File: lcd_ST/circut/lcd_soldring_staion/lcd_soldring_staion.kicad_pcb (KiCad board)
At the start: 2 copper layers, 41.7 x 41 mm, 35 parts, among them J2 Conn_01x05_Pin, J3 Conn_01x01_Pin, J4 Conn_01x01_Pin, J44 Screw_Terminal_01x02, J5 Conn_01x01_Pin, J6 Conn_01x01_Pin, J7 Conn_01x04_Pin, Q2 Si4162DY, SW1 SW_Push, U1 PIC16F15223T-I/SL, U2 L7805, U3 LM358

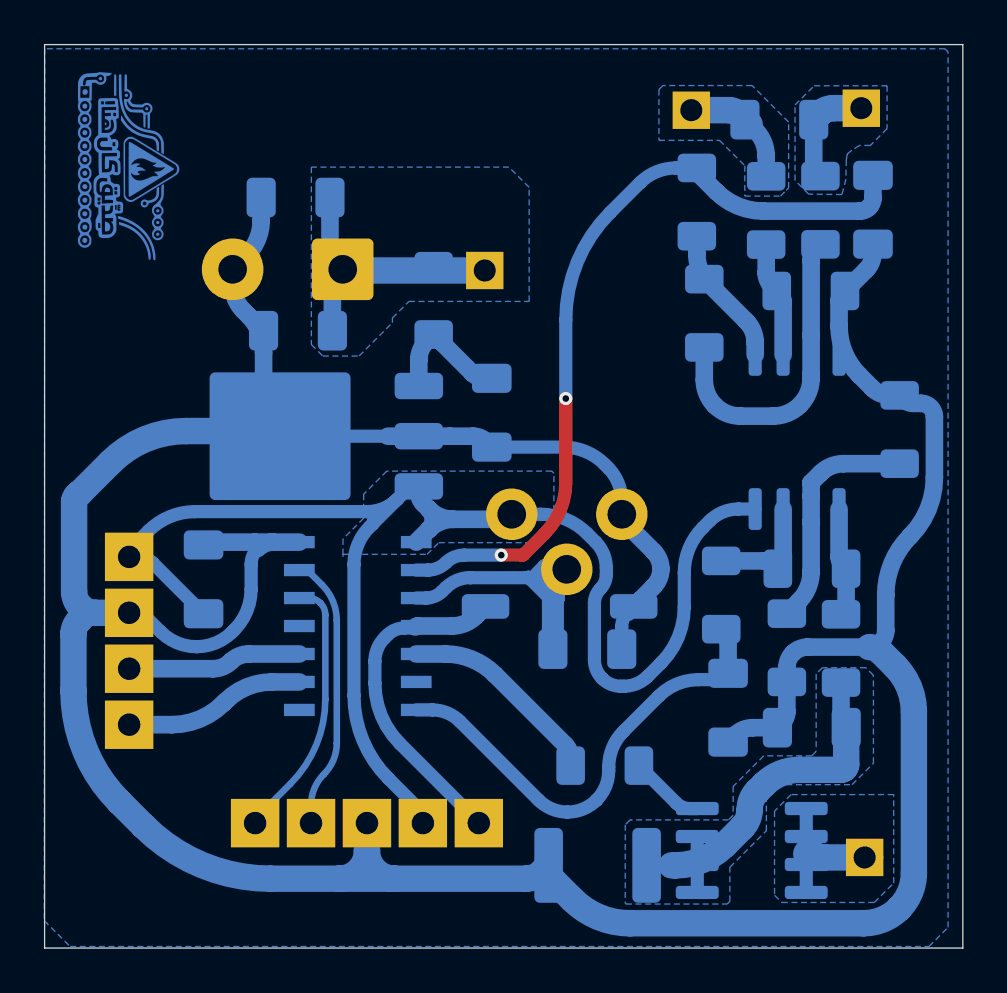
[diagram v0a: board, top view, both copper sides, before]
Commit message: done v0
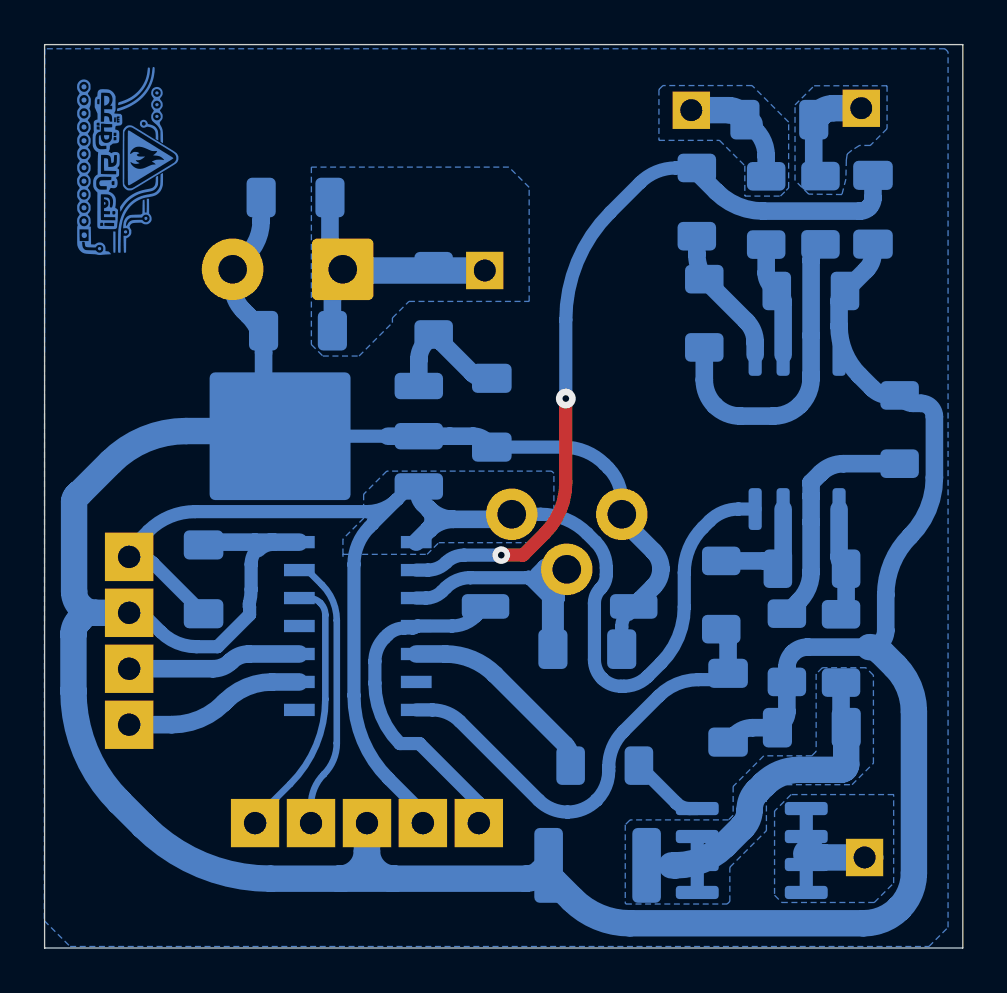
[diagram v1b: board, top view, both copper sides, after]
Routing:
- net VPP: track 15.3 -> 15.8 mm

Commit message: V2_PCB EDITING
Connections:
- C4 pad 1: T+ -> T-
- C4 pad 2: T- -> T+
- C9 pad 1: c+ -> c-
- C9 pad 2: c- -> c+
- R10 pad 2: Net-(U3B--) -> Net-(U3B-+)
- R11 pad 1: Net-(U3B-+) -> Net-(U3B--)
- R2 pad 1: T+ -> T-
- R2 pad 2: Net-(U3A-+) -> Net-(U3A--)
- R3 pad 1: Net-(U3A-+) -> Net-(U3A--)
- R4 pad 1: T- -> T+
- R4 pad 2: Net-(U3A--) -> Net-(U3A-+)
- R5 pad 2: Net-(U3A--) -> Net-(U3A-+)
- R8 pad 1: c+ -> c-
- R8 pad 2: Net-(U3B-+) -> Net-(U3B--)
- R9 pad 1: c- -> c+
- R9 pad 2: Net-(U3B--) -> Net-(U3B-+)
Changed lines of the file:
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@@
 			(layers "B.Cu" "B.Mask" "B.Paste")
 			(roundrect_rratio 0.192308)
-			(net 19 "Net-(U3A--)")
+			(net 17 "Net-(U3A-+)")
 			(pintype "passive")
 		)
@@
 			(layers "B.Cu" "B.Mask" "B.Paste")
 			(roundrect_rratio 0.192308)
-			(net 5 "T-")
+			(net 6 "T+")
 			(pintype "passive")
 		)
@@
 			(layers "B.Cu" "B.Mask" "B.Paste")
 			(roundrect_rratio 0.192308)
-			(net 19 "Net-(U3A--)")
+			(net 17 "Net-(U3A-+)")
 			(pintype "passive")
 		)
@@
 			(layers "B.Cu" "B.Mask" "B.Paste")
 			(roundrect_rratio 0.192308)
-			(net 2 "c-")
+			(net 9 "c+")
 			(pintype "passive")
 		)
@@
 			(layers "B.Cu" "B.Mask" "B.Paste")
 			(roundrect_rratio 0.192308)
-			(net 22 "Net-(U3B--)")
+			(net 21 "Net-(U3B-+)")
 			(pintype "passive")
 		)
@@
 			(layers "B.Cu" "B.Mask" "B.Paste")
 			(roundrect_rratio 0.192308)
-			(net 6 "T+")
+			(net 5 "T-")
 			(pintype "passive")
 		)
@@
 			(layers "B.Cu" "B.Mask" "B.Paste")
 			(roundrect_rratio 0.192308)
-			(net 17 "Net-(U3A-+)")
+			(net 19 "Net-(U3A--)")
 			(pintype "passive")
 		)
@@
 			(layers "B.Cu" "B.Mask" "B.Paste")
 			(roundrect_rratio 0.192308)
-			(net 17 "Net-(U3A-+)")
+			(net 19 "Net-(U3A--)")
 			(pintype "passive")
 		)
@@
 			(layers "B.Cu" "B.Mask" "B.Paste")
 			(roundrect_rratio 0.188679)
-			(net 9 "c+")
+			(net 2 "c-")
 			(pintype "passive")
 		)
@@
 			(layers "B.Cu" "B.Mask" "B.Paste")
 			(roundrect_rratio 0.188679)
-			(net 2 "c-")
+			(net 9 "c+")
 			(pintype "passive")
 		)
@@
 			(layers "B.Cu" "B.Mask" "B.Paste")
 			(roundrect_rratio 0.192308)
-			(net 21 "Net-(U3B-+)")
+			(net 22 "Net-(U3B--)")
 			(pintype "passive")
 		)
@@
 			(layers "B.Cu" "B.Mask" "B.Paste")
 			(roundrect_rratio 0.192308)
-			(net 22 "Net-(U3B--)")
+			(net 21 "Net-(U3B-+)")
 			(pintype "passive")
 		)
@@
 			(layers "B.Cu" "B.Mask" "B.Paste")
 			(roundrect_rratio 0.188679)
-			(net 6 "T+")
+			(net 5 "T-")
 			(pintype "passive")
 		)
@@
 			(layers "B.Cu" "B.Mask" "B.Paste")
 			(roundrect_rratio 0.188679)
-			(net 5 "T-")
+			(net 6 "T+")
 			(pintype "passive")
 		)
@@
 			(layers "B.Cu" "B.Mask" "B.Paste")
 			(roundrect_rratio 0.192308)
-			(net 9 "c+")
+			(net 2 "c-")
 			(pintype "passive")
 		)
@@
 			(layers "B.Cu" "B.Mask" "B.Paste")
 			(roundrect_rratio 0.192308)
-			(net 21 "Net-(U3B-+)")
+			(net 22 "Net-(U3B--)")
 			(pintype "passive")
 		)
